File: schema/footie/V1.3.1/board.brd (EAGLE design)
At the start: 46.1 x 48.9 mm, 44 parts, among them T1 2N3565, U1 IRLML2246TRPBF, U2 USD-SOCKETNEW, U4 MCP73831, U5 3.3 regulator, U6 ATMEGA328P-AU

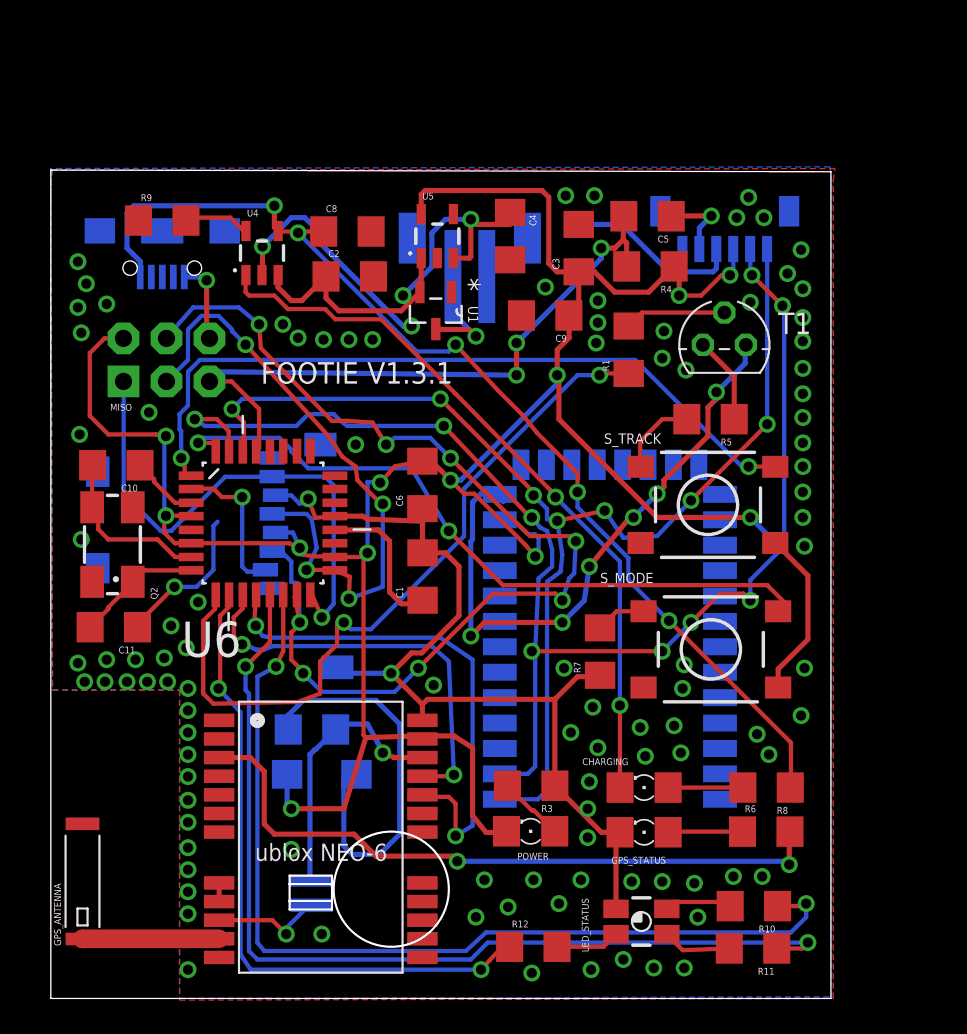
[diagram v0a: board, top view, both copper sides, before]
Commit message: complete board but not happy
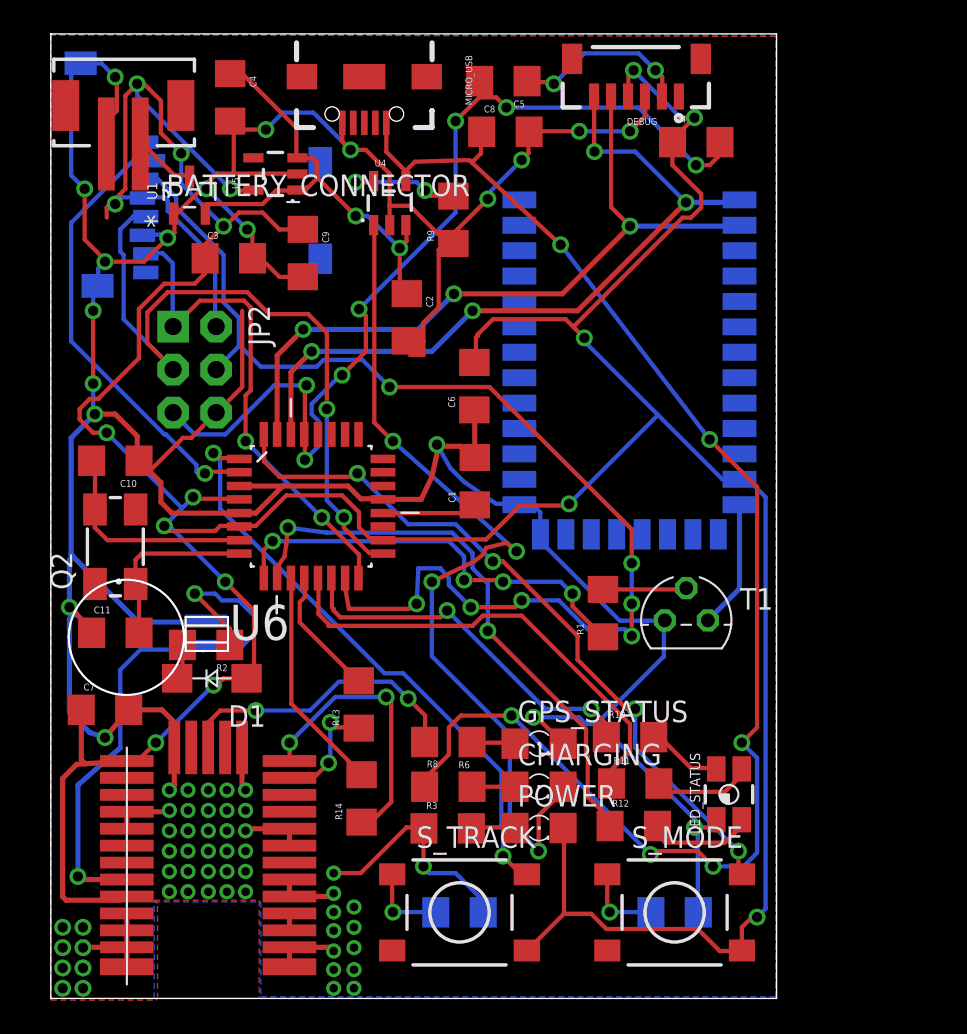
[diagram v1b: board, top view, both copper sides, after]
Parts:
- removed GPS_ANTENNA: ANTENNA2SMD6, SparkFun-RF:ANTENNA-CHIP6
- removed U$1: UBLOX_NEO-6, Ava:UBLOX_NEO-6P
- added C7: 4.7 uF, SparkFun-Capacitors:1206
- added R13, R14: 220 Ohm, SparkFun-Passives:1206
- added U3: CAM-M8Q, CAM-M8Q:CAM-M8Q
- moved BLUETOOTH 38.1 mm to (40.7, 47.1), turned to 0 degrees
- moved R5 32.7 mm to (24.1, 5.08), flipped to the bottom, turned to 0 degrees
- moved S_TRACK 28.2 mm to (24.1, 5.08)
- moved BATTERY_CONNECTOR 21.9 mm to (4.28, 52.5), flipped to the top
- moved C3 20.7 mm to (10.5, 43.7), turned to 0 degrees
- moved R6 19.5 mm to (23.5, 15.1), turned to 180 degrees
- moved R8 18.8 mm to (23.5, 12.5), turned to 0 degrees
- moved C4 18.4 mm to (10.6, 53.2)
- moved R9 17.2 mm to (23.8, 46.0), turned to 90 degrees
- moved T1 16.4 mm to (37.5, 22.3)
- moved U2 16.3 mm to (16.3, 41.6), turned to 270 degrees
- moved U1 16.1 mm to (8.19, 47.4), turned to 90 degrees
- moved R7 16.0 mm to (36.8, 5.08), flipped to the bottom, turned to 0 degrees
- moved S_MODE 15.7 mm to (36.8, 5.08)
- moved R1 15.6 mm to (32.6, 22.8)
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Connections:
- removed net N$6 (its old number): R2.1, U$1.22_V_BCKP, U$3.3V
- removed net N$7: GPS_ANTENNA.1, U$1.11_RF_IN
- removed net SCL: U$1.19_SCL2
- removed net SDA: U$1.18_SDA2
- new net N$25: R13.1, U3.25
- new net N$26: R14.1, U3.26
- new net N$4: R6.2, U3.29
- net +3V3: now also C7.1, U3.1, U3.9; no longer U$1.23_VCC
- net GND: now also C7.2, U3.10, U3.11, U3.12, U3.13, U3.14, U3.15, U3.18, U3.19, U3.21, U3.22, U3.27, U3.31, U3.4, U3.5; no longer U$1.10_GND, U$1.12_GND, U$1.13_GND, U$1.24_GND, U$1.7_VDDUSB
- net GPSRX: now also R14.2; no longer U$1.21_RXD1
- net GPSTX: now also R13.2; no longer U$1.20_TXD1
- net N$3: now also U3.16, U3.17; no longer R6.2, U$1.3_TIMEPULSE
- net N$5: now also R2.1, U$3.3V, U3.8; no longer U$1.8_RESERVED, U$1.9_VCC_RF
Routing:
- net GND: track 111.9 -> 280.7 mm, vias 108 -> 71
- net +3V3: track 160.4 -> 245.0 mm, vias 12 -> 16
- net N$3: track 40.1 -> 1.00 mm, vias 2 -> 0
- net ARDUINO_TX: track 81.3 -> 43.3 mm, vias 9 -> 3
- net D10: track 57.3 -> 22.0 mm
- net N$5: track 1.10 -> 35.1 mm, vias 0 -> 2
- net N$20: track 37.9 -> 7.60 mm, vias 6 -> 0
- net D9: track 57.3 -> 27.7 mm, vias 2 -> 0
- net ARDUINO_RX: track 71.4 -> 44.3 mm, vias 7 -> 4
- net GPSTX: track 30.4 -> 7.66 mm, vias 2 -> 0
- net N$1: track 23.8 -> 2.10 mm
- net N$2: track 64.0 -> 84.9 mm, vias 5 -> 6
- net DTR: track 38.7 -> 58.4 mm, vias 3 -> 7
- net SD_CS: track 8.87 -> 26.8 mm
- net D5: track 43.3 -> 25.5 mm, vias 2 -> 4
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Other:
- board size 46.1 x 48.9 mm -> 42.9 x 57 mm
- board text removed: "FOOTIE V1.3.1"
- board text removed: "MISO"

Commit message: update version, bit bigger but better design
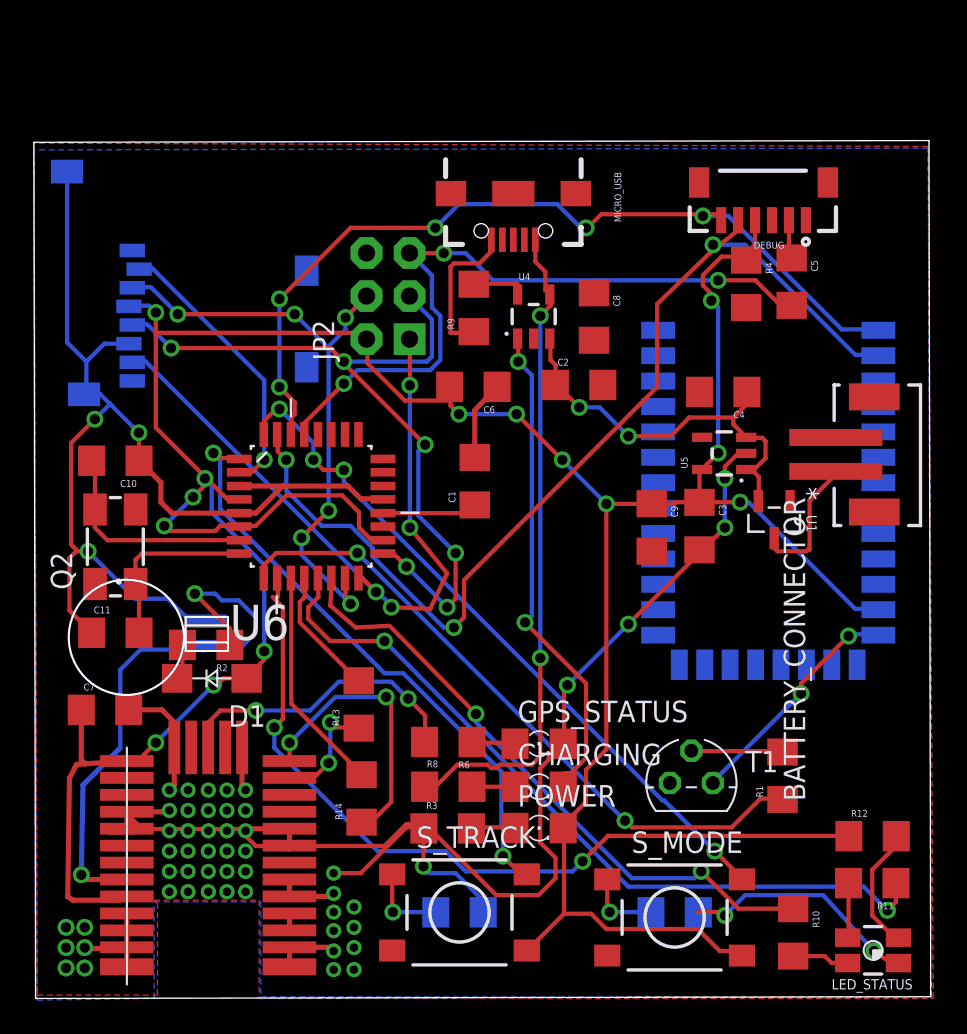
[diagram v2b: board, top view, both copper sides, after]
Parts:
- moved BATTERY_CONNECTOR 48.5 mm to (48.4, 32.1), turned to 270 degrees
- moved U1 39.5 mm to (42.7, 28.3), turned to 270 degrees
- moved C4 33.9 mm to (39.7, 35.8), turned to 180 degrees
- moved C3 32.0 mm to (38.3, 27.9), turned to 270 degrees
- moved U5 31.2 mm to (39.8, 32.2)
- moved C9 26.2 mm to (35.5, 27.8)
- moved C5 20.7 mm to (43.7, 42.3), turned to 270 degrees
- moved R11 15.2 mm to (48.5, 6.81), turned to 180 degrees
- moved R10 15.0 mm to (43.8, 3.90), turned to 270 degrees
- moved R1 14.3 mm to (43.2, 13.2)
- moved R12 14.1 mm to (48.5, 9.58)
- moved LED_STATUS 12.5 mm to (48.5, 2.84), turned to 270 degrees
- moved JP2 12.2 mm to (19.9, 41.5), turned to 90 degrees
- moved C8 12.1 mm to (32.1, 40.3), turned to 270 degrees
- moved BLUETOOTH 11.2 mm to (48.9, 39.5)
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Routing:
- net GND: track 280.7 -> 203.3 mm, vias 71 -> 56
- net +3V3: track 245.0 -> 187.5 mm, vias 16 -> 14
- net N$2: track 84.9 -> 39.1 mm, vias 6 -> 2
- net SD_MOSI: track 71.7 -> 35.7 mm, vias 7 -> 6
- net N$11: track 52.2 -> 29.2 mm, vias 4 -> 2
- net ARDUINO_TX: track 43.3 -> 62.0 mm
- net D9: track 27.7 -> 45.8 mm, vias 0 -> 2
- net DTR: track 58.4 -> 41.2 mm, vias 7 -> 3
- net D10: track 22.0 -> 37.0 mm
- net D6: track 34.0 -> 48.8 mm
- net D5: track 25.5 -> 39.1 mm, vias 4 -> 2
- net SD_MISO: track 29.8 -> 42.0 mm, vias 2 -> 4
- net SD_CS: track 26.8 -> 16.6 mm
- net N$13: track 10.5 -> 2.30 mm, vias 2 -> 0
- net ARDUINO_RX: track 44.3 -> 51.3 mm, vias 4 -> 5
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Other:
- board size 42.9 x 57 mm -> 53 x 50.6 mm
